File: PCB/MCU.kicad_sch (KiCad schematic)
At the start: 31 parts, among them J1 SWD, SW68 Reset, SW69 BOOT_SEL, U1 RP2040, U2 W25Q128JVS, U3 SN74AHCT1G125, Y1 12MHz

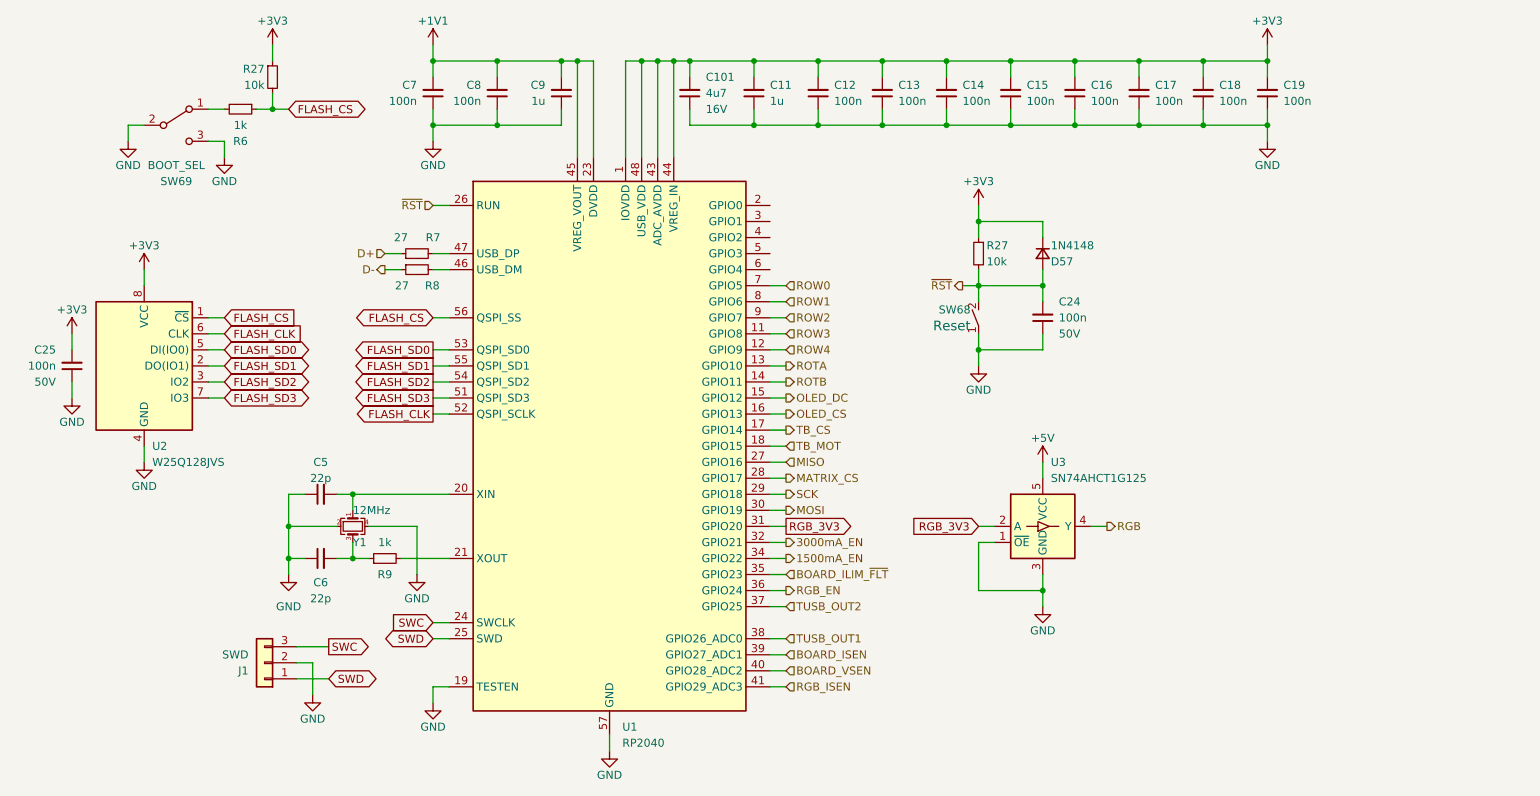
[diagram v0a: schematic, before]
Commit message: BLE version incomplete update.
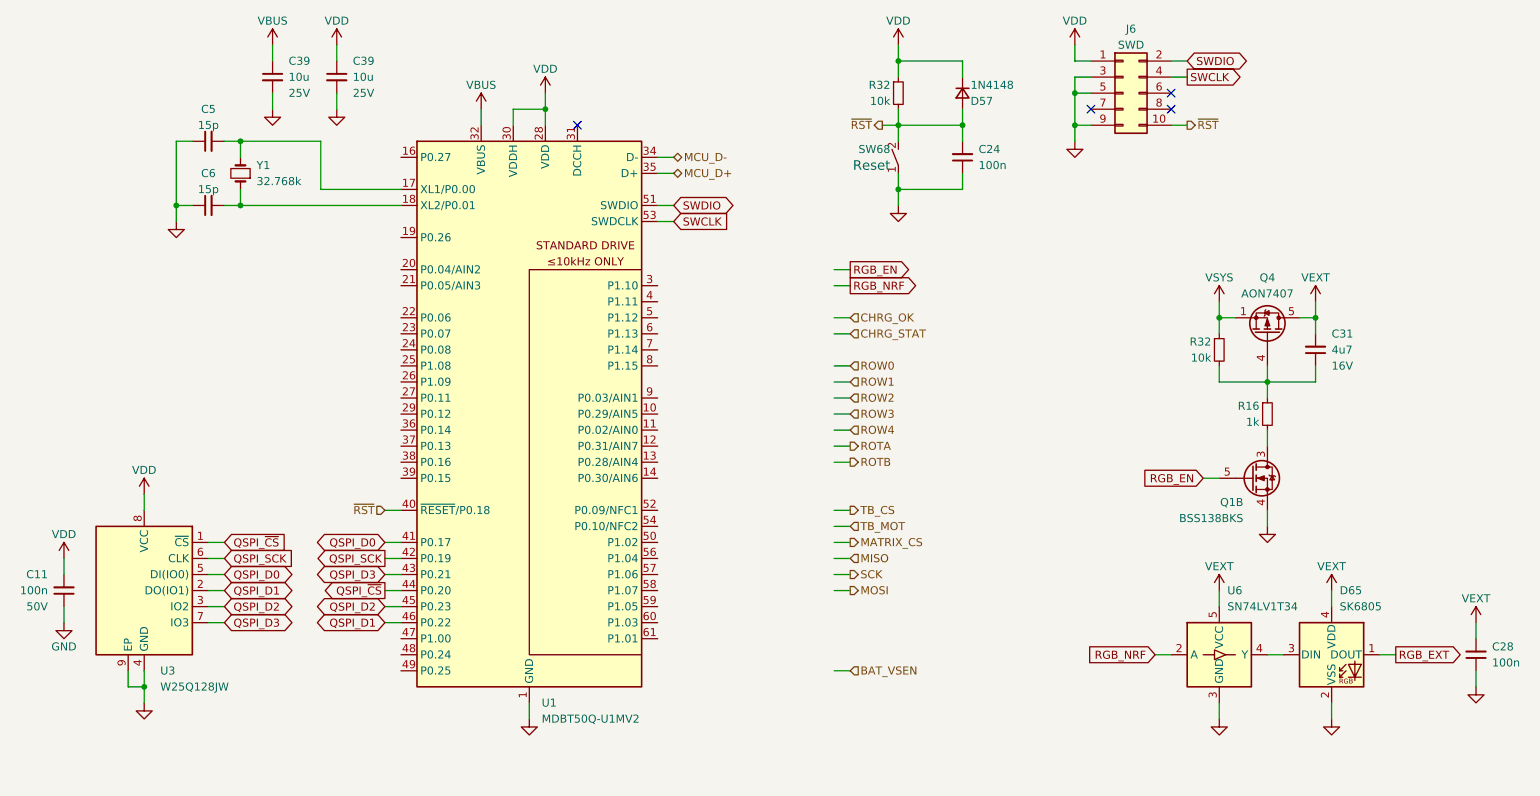
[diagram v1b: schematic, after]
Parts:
- removed C101: 4u7, Capacitor_SMD:C_0603_1608Metric, symbol Device:C_Small
- removed C12, C13, C14, C15, C16, C17, C18, C19, C25, C7, C8: 100n, Capacitor_SMD:C_0402_1005Metric, symbol Device:C_Small
- removed C9: 1u, Capacitor_SMD:C_0603_1608Metric, symbol Device:C_Small
- removed J1: SWD, Honeydew:Header_SWD, symbol Connector_Generic:Conn_01x03
- removed R27 (x2): 10k, Resistor_SMD:R_0402_1005Metric, symbol Device:R_Small
- removed R6, R9: 1k, Resistor_SMD:R_0402_1005Metric, symbol Device:R_Small
- removed R7, R8: 27, Resistor_SMD:R_0402_1005Metric, symbol Device:R_Small
- removed SW69: BOOT_SEL, Button_Switch_SMD:SW_SPDT_PCM12, symbol Switch:SW_SPDT
- removed U1: RP2040, Honeydew:QFN-56-1EP_7x7mm_P0.4mm_EP3.2x3.2mm_ThermalVias, symbol MCU_RaspberryPi:RP2040
- removed U2: W25Q128JVS, Honeydew:SOIC-8_5.23x5.23mm_P1.27mm, symbol Memory_Flash:W25Q128JVS
- removed U3: SN74AHCT1G125, Package_TO_SOT_SMD:SOT-23-5, symbol Honeydew:SN74AHCT1G125
- removed Y1: 12MHz, Crystal:Crystal_SMD_3225-4Pin_3.2x2.5mm, symbol Device:Crystal_GND24_Small
- added C28: 100n, Capacitor_SMD:C_0402_1005Metric, symbol Device:C_Small
- added C31: 4u7, Capacitor_SMD:C_0603_1608Metric, symbol Device:C_Small
- added C39 (x2): 10u, Capacitor_SMD:C_0603_1608Metric, symbol Device:C_Small
- added D65: SK6805, LED_SMD:LED_SK6805_PLCC4_2.4x2.7mm_P1.3mm, symbol LED:SK6805
- added J6: SWD, Connector_PinHeader_1.27mm:PinHeader_2x05_P1.27mm_Vertical, symbol Connector_Generic:Conn_02x05_Odd_Even
- added Q1: BSS138BKS, Package_TO_SOT_SMD:SOT-363_SC-70-6, symbol Device:Q_Dual_NMOS_S1G1D2S2G2D1
- added Q4: AON7407, Honeydew:AO_DFN-8-3x3, symbol Transistor_FET:AON6411
- added R16: 1k, Resistor_SMD:R_0402_1005Metric, symbol Device:R_Small
- added R32 (x2): 10k, Resistor_SMD:R_0402_1005Metric, symbol Device:R_Small
- added U1: MDBT50Q-U1MV2, RF_Module:Raytac_MDBT50Q, symbol Honeydew:MDBT50Q
- added U3: W25Q128JW, Package_SON:WSON-8-1EP_6x5mm_P1.27mm_EP3.4x4.3mm, symbol Memory_Flash:W25Q32JVZP
- added U6: SN74LV1T34, Package_TO_SOT_SMD:SOT-353_SC-70-5, symbol Logic_LevelTranslator:SN74LV1T34DCK
- added Y1: 32.768k, Crystal:Crystal_SMD_3215-2Pin_3.2x1.5mm, symbol Device:Crystal_Small
- C11: value 1u -> 100n; footprint Capacitor_SMD:C_0603_1608Metric -> Capacitor_SMD:C_0402_1005Metric; LCSC C15849 -> C307331
- C5, C6: value 22p -> 15p; LCSC C1555 -> C1548
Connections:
- net GND: now also C28.1, C39.2, C39.2, D65.2 (VSS), J6.3 (Pin_3), J6.5 (Pin_5), J6.9 (Pin_9), Q1.4 (S), U1.1 (GND), U1.15 (GND), U1.2 (GND), U1.33 (GND), U1.55 (GND), U3.4 (GND), U3.9 (EP), U6.3 (GND)
- net RGB_EN: now also Q1.5 (G)
- net ~{RST}: now also J6.10 (Pin_10), R32.2, U1.40 (~{RESET}/P0.18)
- net at C6.2: now also U1.18 (XL2/P0.01), Y1.1
- net at C5.2: now also U1.17 (XL1/P0.00), Y1.2
- net +3V3 renamed VDD
- net VDD: now also C39.1, J6.1 (Pin_1), R32.1, U1.28 (VDD), U1.30 (VDDH), U3.8 (VCC)
- new net: D65.3 (DIN), U6.4 (Y)
- new net: C31.1, Q4.4 (G), R16.1, R32.2
- new net: Q1.3 (D), R16.2
- new net MCU_D+: U1.35 (D+)
- new net MCU_D-: U1.34 (D-)
- new net QSPI_D0: U1.41 (P0.17), U3.5 (DI(IO0))
- new net QSPI_D1: U1.46 (P0.22), U3.2 (DO(IO1))
- new net QSPI_D2: U1.45 (P0.23), U3.3 (IO2)
- new net QSPI_D3: U1.43 (P0.21), U3.7 (IO3)
- new net QSPI_SCK: U1.42 (P0.19), U3.6 (CLK)
- new net QSPI_~{CS}: U1.44 (P0.20), U3.1 (~{CS})
- new net RGB_EXT: D65.1 (DOUT)
- new net RGB_NRF: U6.2 (A)
- new net SWCLK: J6.4 (Pin_4), U1.53 (SWDCLK)
- new net SWDIO: J6.2 (Pin_2), U1.51 (SWDIO)
- new net VBUS: C39.1, U1.32 (VBUS)
- new net VEXT: C28.2, C31.2, D65.4 (VDD), Q4.5 (D), U6.5 (VCC)
- new net VSYS: Q4.1 (S), Q4.2 (S), Q4.3 (S), R32.1
- no-connect marks 0 -> 4
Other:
- moved on the sheet: C24, D57, SW68
